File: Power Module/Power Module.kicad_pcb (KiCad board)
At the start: 2 copper layers, 89.2 x 84.8 mm, 123 parts, among them J1 Conn_02x14_Odd_Even, J2 MOTOR, J3 MOTOR, J4 MOTOR, J5 MOTOR, Q1 CSD18509Q5B, Q10 CSD18509Q5B, Q11 CSD18509Q5B, Q12 CSD18509Q5B, Q13 CSD18509Q5B, Q14 CSD18509Q5B, Q15 CSD18509Q5B, Q16 CSD18509Q5B, Q17 CSD18509Q5B, Q18 CSD18509Q5B, Q19 CSD18509Q5B, Q2 CSD18509Q5B, Q20 CSD18509Q5B, Q21 CSD18509Q5B, Q22 CSD18509Q5B, Q23 CSD18509Q5B, Q24 CSD18509Q5B, Q3 CSD18509Q5B, Q4 CSD18509Q5B, Q5 CSD18509Q5B, Q6 CSD18509Q5B, Q7 CSD18509Q5B, Q8 CSD18509Q5B, Q9 CSD18509Q5B, U1 LM2576S-3.3, U2 MCF8329A1IREER, U3 MCF8329A1IREER, U4 MCF8329A1IREER, U5 MCF8329A1IREER, U6 TCA9548APWR

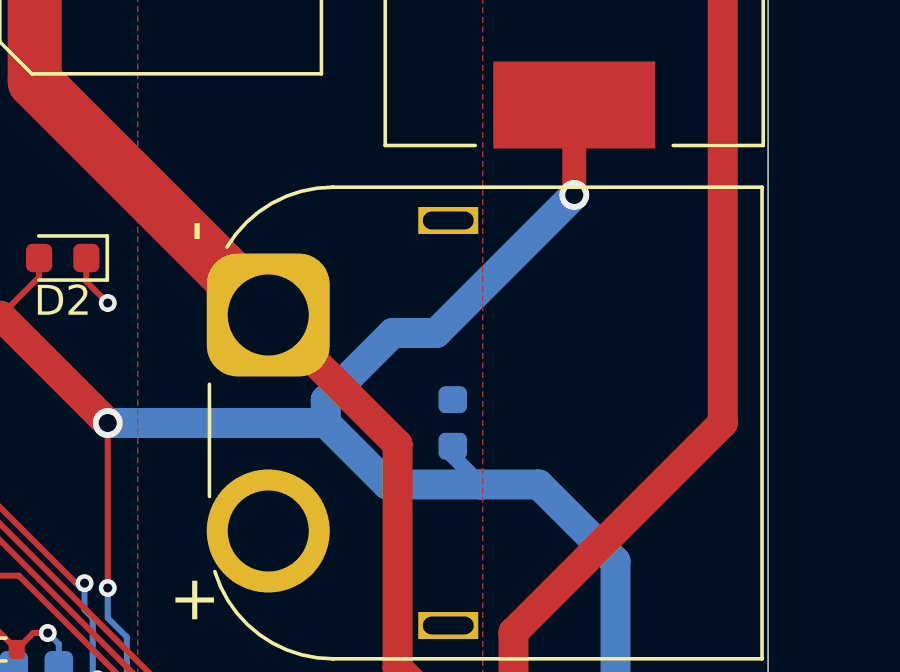
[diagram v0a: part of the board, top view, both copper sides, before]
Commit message: More localization work
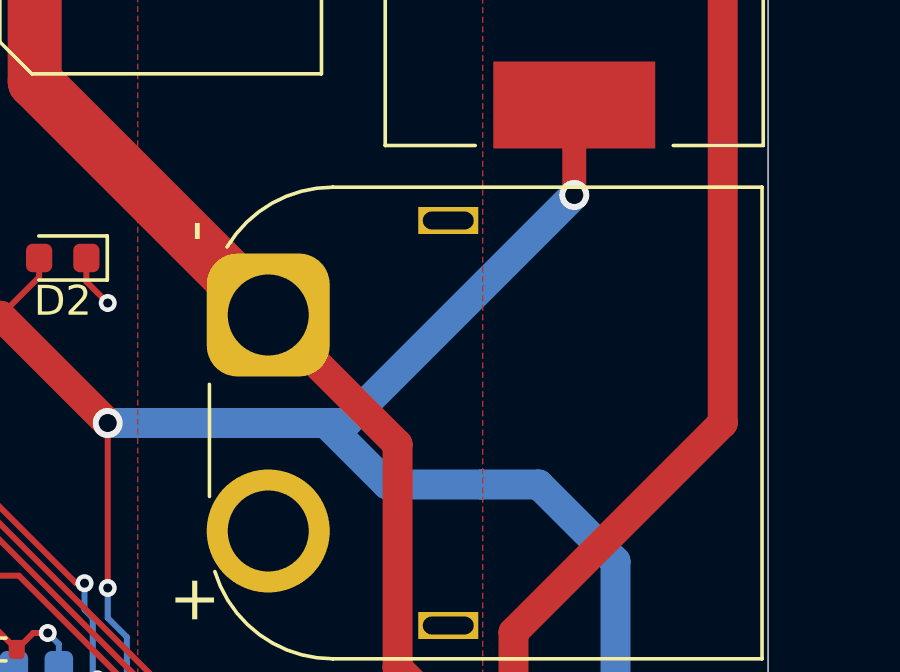
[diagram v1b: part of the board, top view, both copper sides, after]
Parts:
- removed C2: 1000uF, Capacitor_SMD:C_0603_1608Metric
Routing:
- net +3V3: track 306.5 -> 304.4 mm
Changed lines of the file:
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@@
 		(tags "resistor")
 		(property "Reference" "R33"
-			(at 0 1.17 360)
+			(at 0 1.17 0)
 			(layer "B.SilkS")
 			(effects
@@
 		)
 		(property "Value" "4.7k"
-			(at 0 -1.17 360)
+			(at 0 -1.17 0)
 			(layer "B.Fab")
 			(effects
@@
 		)
 		(fp_text user "${REFERENCE}"
-			(at 0 0 360)
+			(at 0 0 0)
 			(layer "B.Fab")
 			(effects
@@
 		)
 	)
-	(footprint "Capacitor_SMD:C_0603_1608Metric"
-		(layer "B.Cu")
-		(at 127.5 83.5 90)
-		(descr "Capacitor SMD 0603 (1608 Metric), square (rectangular) end terminal, IPC_7351 nominal, (Body size source: IPC-SM-782 page 76, https://www.pcb-3d.com/wordpress/wp-content/uploads/ipc-sm-782a_amendment_1_and_2.pdf), generated with kicad-footprint-generator")
-		(tags "capacitor")
-		(property "Reference" "C2"
-			(at 0 1.43 90)
-			(layer "B.SilkS")
-			(effects
-				(font
-					(size 1 1)
-					(thickness 0.15)
-				)
-				(justify mirror)
-			)
-		)
-		(property "Value" "1000uF"
-			(at 0 -1.43 90)
-			(layer "B.Fab")
-			(effects
-				(font
-					(size 1 1)
-					(thickness 0.15)
-				)
-				(justify mirror)
-			)
-		)
-		(property "Footprint" "Capacitor_SMD:C_0603_1608Metric"
-			(at 0 0 -90)
-			(unlocked yes)
-			(layer "B.Fab")
-			(hide yes)
-			(effects
-				(font
-					(size 1.27 1.27)
-					(thickness 0.15)
-				)
-				(justify mirror)
-			)
-		)
-		(property "Datasheet" ""
-			(at 0 0 -90)
-			(unlocked yes)
-			(layer "B.Fab")
-			(hide yes)
-			(effects
-				(font
-					(size 1.27 1.27)
-					(thickness 0.15)
-				)
-				(justify mirror)
-			)
-		)
-		(property "Description" "Unpolarized capacitor"
-			(at 0 0 -90)
-			(unlocked yes)
-			(layer "B.Fab")
-			(hide yes)
-			(effects
-				(font
-					(size 1.27 1.27)
-					(thickness 0.15)
-				)
-				(justify mirror)
-			)
-		)
-		(property ki_fp_filters "C_*")
-		(sheetname "Root")
-		(sheetfile "Power Module.kicad_sch")
-		(attr smd)
-		(fp_line
-			(start 0.14058 -0.51)
-			(end -0.14058 -0.51)
-			(stroke
-				(width 0.12)
-				(type solid)
-			)
-			(layer "B.SilkS")
-		)
-		(fp_line
-			(start 0.14058 0.51)
-			(end -0.14058 0.51)
-			(stroke
-				(width 0.12)
-				(type solid)
-			)
-			(layer "B.SilkS")
-		)
-		(fp_line
-			(start 1.48 -0.73)
-			(end 1.48 0.73)
-			(stroke
-				(width 0.05)
-				(type solid)
-			)
-			(layer "B.CrtYd")
-		)
-		(fp_line
-			(start -1.48 -0.73)
-			(end 1.48 -0.73)
-			(stroke
-				(width 0.05)
-				(type solid)
-			)
-			(layer "B.CrtYd")
-		)
-		(fp_line
-			(start 1.48 0.73)
-			(end -1.48 0.73)
-			(stroke
-				(width 0.05)
-				(type solid)
-			)
-			(layer "B.CrtYd")
-		)
-		(fp_line
-			(start -1.48 0.73)
-			(end -1.48 -0.73)
-			(stroke
-				(width 0.05)
-				(type solid)
-			)
-			(layer "B.CrtYd")
-		)
-		(fp_line
-			(start 0.8 -0.4)
-			(end 0.8 0.4)
-			(stroke
-				(width 0.1)
-				(type solid)
-			)
-			(layer "B.Fab")
-		)
-		(fp_line
-			(start -0.8 -0.4)
-			(end 0.8 -0.4)
-			(stroke
-				(width 0.1)
-				(type solid)
-			)
-			(layer "B.Fab")
-		)
-		(fp_line
-			(start 0.8 0.4)
-			(end -0.8 0.4)
-			(stroke
-				(width 0.1)
-				(type solid)
-			)
-			(layer "B.Fab")
-		)
-		(fp_line
-			(start -0.8 0.4)
-			(end -0.8 -0.4)
-			(stroke
-				(width 0.1)
-				(type solid)
-			)
-			(layer "B.Fab")
-		)
-		(fp_text user "${REFERENCE}"
-			(at 0 0 90)
-			(layer "B.Fab")
-			(effects
-				(font
-					(size 0.4 0.4)
-					(thickness 0.06)
-				)
-				(justify mirror)
-			)
-		)
-		(pad "1" smd roundrect
-			(at -0.775 0 90)
-			(size 0.9 0.95)
-			(layers "B.Cu" "B.Paste" "B.Mask")
-			(roundrect_rratio 0.25)
-			(net 3 "+3V3")
-			(pintype "passive")
-		)
-		(pad "2" smd roundrect
-			(at 0.775 0 90)
-			(size 0.9 0.95)
-			(layers "B.Cu" "B.Paste" "B.Mask")
-			(roundrect_rratio 0.25)
-			(net 2 "AGND")
-			(pintype "passive")
-		)
-		(model "${KICAD8_3DMODEL_DIR}/Capacitor_SMD.3dshapes/C_0603_1608Metric.wrl"
-			(offset
-				(xyz 0 0 0)
-			)
-			(scale
-				(xyz 1 1 1)
-			)
-			(rotate
-				(xyz 0 0 0)
-			)
-		)
-	)
 	(footprint "Resistor_SMD:R_0603_1608Metric_Pad0.98x0.95mm_HandSolder"
 		(layer "B.Cu")
@@
 	)
 	(segment
-		(start 125.5 80.5)
-		(end 126.95 80.5)
-		(width 1)
-		(layer "B.Cu")
-		(net 3)
-	)
-	(segment
 		(start 130.365831 85.55)
 		(end 128.45 85.55)
@@
 	)
 	(segment
-		(start 123.267084 82.732916)
-		(end 123.267084 83.5)
-		(width 1)
-		(layer "B.Cu")
-		(net 3)
-	)
-	(segment
 		(start 116.635485 91.5)
 		(end 116.635485 90.635485)
@@
 	)
 	(segment
-		(start 127.5 84.6)
-		(end 128.45 85.55)
-		(width 0.5)
-		(layer "B.Cu")
-		(net 3)
-	)
-	(segment
 		(start 116.333063 92.635)
 		(end 117.5 93.801937)
@@
 	)
 	(segment
-		(start 126.95 80.5)
-		(end 131.55 75.9)
-		(width 1)
-		(layer "B.Cu")
-		(net 3)
-	)
-	(segment
 		(start 80.793735 91.5875)
 		(end 80.286235 91.08)
@@
 	)
 	(segment
+		(start 123.95 83.5)
+		(end 123.267084 83.5)
+		(width 1)
+		(layer "B.Cu")
+		(net 3)
+	)
+	(segment
 		(start 90 80.925)
 		(end 91 79.925)
@@
 	)
 	(segment
-		(start 127.5 84.275)
-		(end 127.5 84.6)
-		(width 0.5)
-		(layer "B.Cu")
-		(net 3)
-	)
-	(segment
 		(start 72.5 77)
 		(end 72.5 79.925)
@@
 	)
 	(segment
-		(start 125.317084 85.55)
-		(end 123.267084 83.5)
+		(start 131.55 75.9)
+		(end 123.95 83.5)
 		(width 1)
 		(layer "B.Cu")
@@
 	)
 	(segment
-		(start 125.5 80.5)
-		(end 123.267084 82.732916)
+		(start 125.317084 85.55)
+		(end 123.267084 83.5)
 		(width 1)
 		(layer "B.Cu")
